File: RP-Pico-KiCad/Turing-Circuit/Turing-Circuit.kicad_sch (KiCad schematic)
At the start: 16 parts

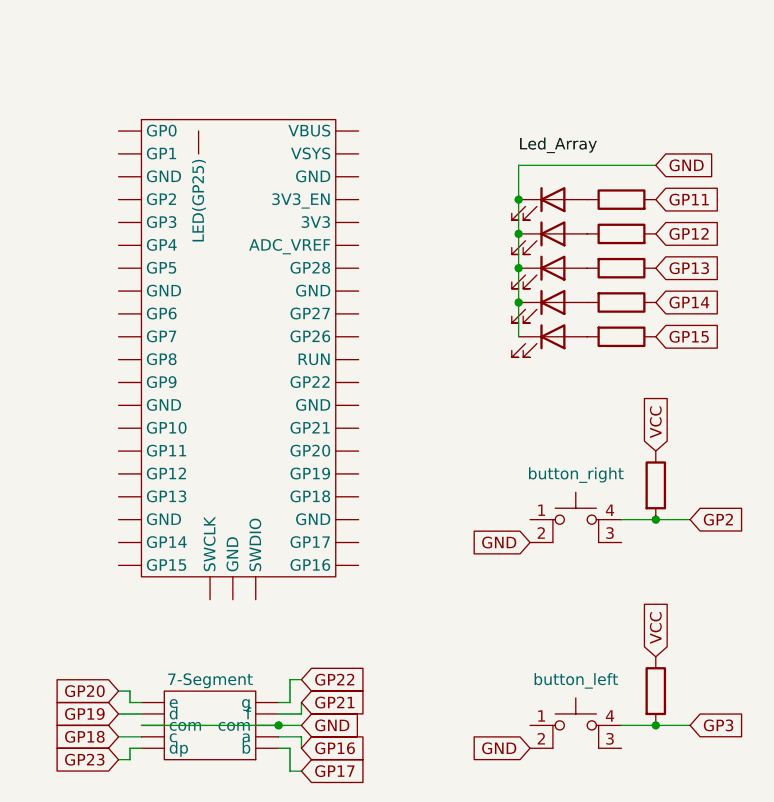
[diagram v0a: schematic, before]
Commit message: bugfixes and schematic
adding ciruit schematic for project
bux fixes
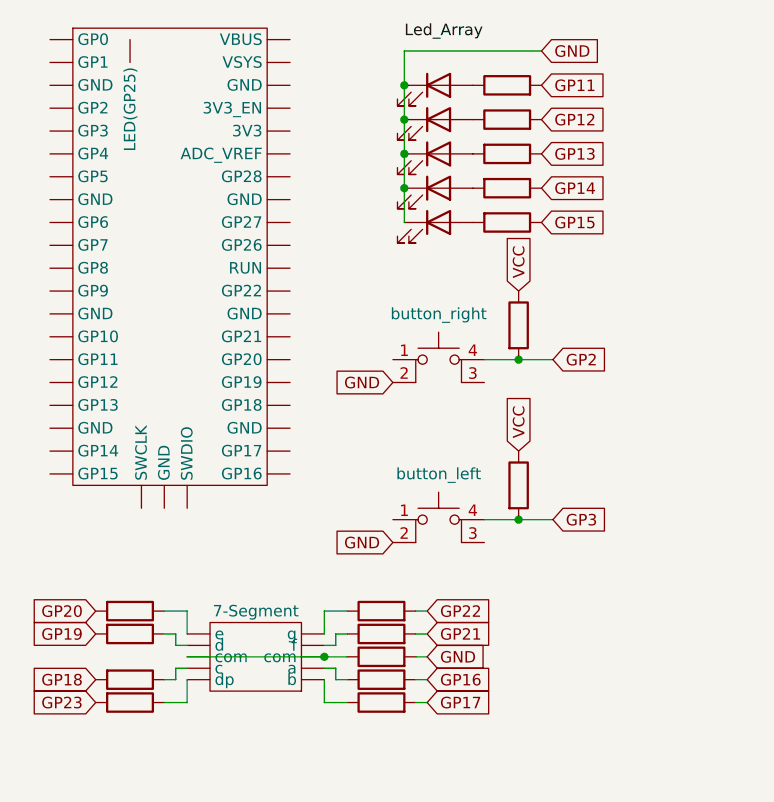
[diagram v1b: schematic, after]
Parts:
- added R10, R11, R12, R13, R14, R16, R17, R8, R9: R, symbol Device:R
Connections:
- net GND: now also R12.2; no longer 7-Segment1. (g)
- net GP16: now also R9.2; no longer 7-Segment1. (g)
- net GP17: now also R8.2; no longer 7-Segment1. (g)
- net GP18: now also R14.2; no longer 7-Segment1. (g)
- net GP19: now also R16.2; no longer 7-Segment1. (g)
- net GP20: now also R17.2; no longer 7-Segment1. (g)
- net GP21: now also R11.2; no longer 7-Segment1. (g)
- net GP22: now also R10.2; no longer 7-Segment1. (g)
- net GP23: now also R13.2; no longer 7-Segment1. (g)
- new net: 7-Segment1. (g), R12.1
- new net: 7-Segment1. (g), R10.1
- new net: 7-Segment1. (g), R8.1
- new net: 7-Segment1. (g), R13.1
- new net: 7-Segment1. (g), R16.1
- new net: 7-Segment1. (g), R17.1
- new net: 7-Segment1. (g), R9.1
- new net: 7-Segment1. (g), R14.1
- new net: 7-Segment1. (g), R11.1
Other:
- moved on the sheet: button_left, button_right
